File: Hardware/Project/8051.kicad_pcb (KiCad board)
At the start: 2 copper layers, 48 parts, among them J1 USB_B_Mini, J2 Conn_02x20_Odd_Even, Q1 9015, Q2 9013, SW1 reset, U1 8255, U10 74LS138, U11 74LS14, U12 74LS00, U13 STC89C52-Vintage, U14 74LS08, U18 74LS32, U19 74LS30, U2 74LS373_ARRANGED, U20 AT29C512, U21 74LS32, U22 74LS138, U5 74LS138, U6 28C256, U7 28C256, U9 ATA, Y2 Crystal

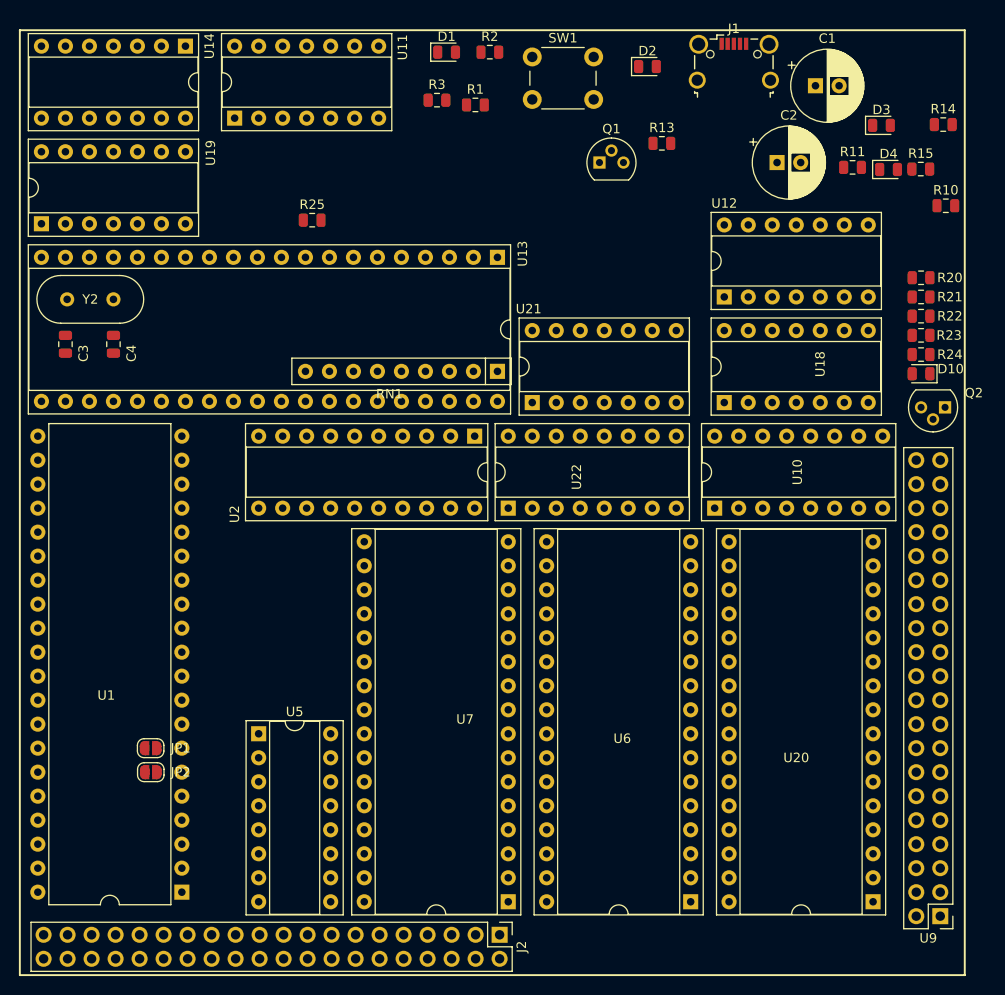
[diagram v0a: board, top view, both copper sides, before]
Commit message: 1
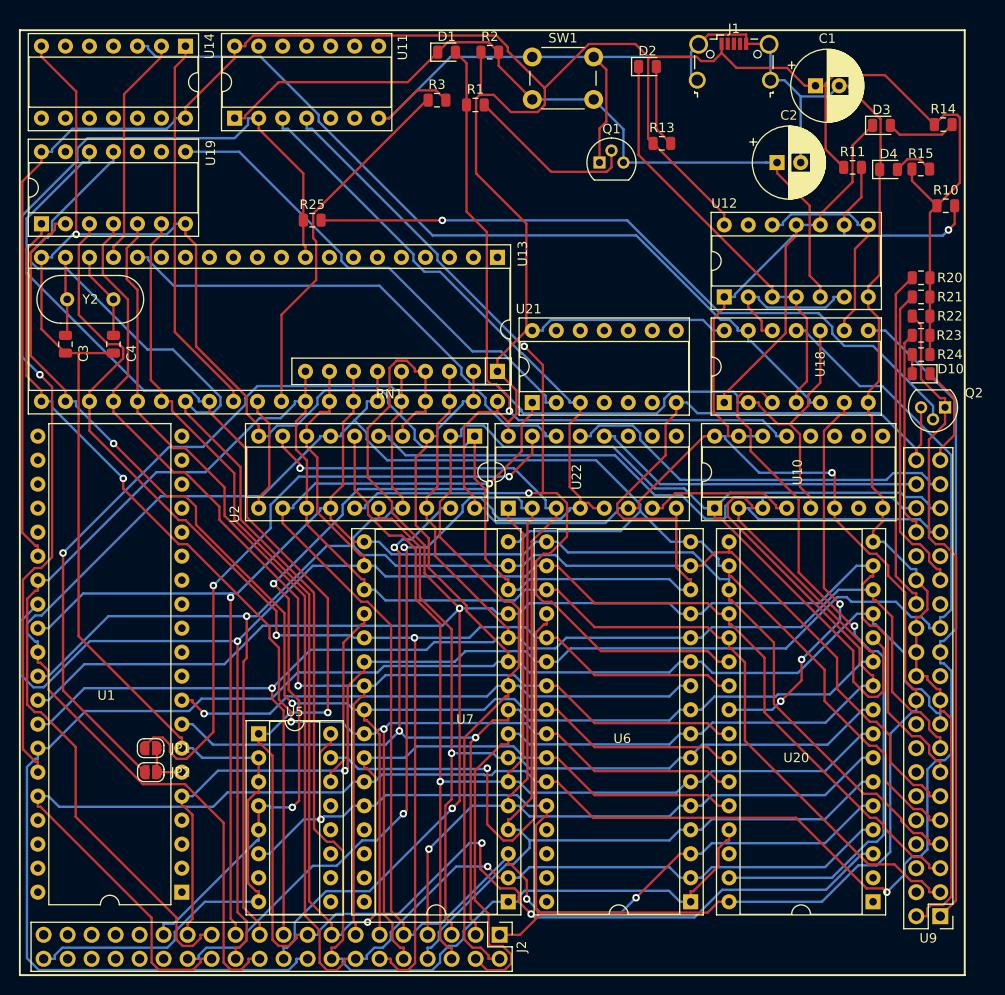
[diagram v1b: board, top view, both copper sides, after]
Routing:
- net /+5V: track 0.00 -> 506.3 mm, vias 0 -> 2
- net /GND: track 0.00 -> 502.7 mm, vias 0 -> 1
- net /~A0: track 0.00 -> 214.9 mm, vias 0 -> 1
- net /~D2: track 0.00 -> 214.0 mm, vias 0 -> 2
- net /~D0: track 0.00 -> 204.2 mm
- net /~D4: track 0.00 -> 203.5 mm
- net /~WR: track 0.00 -> 197.2 mm, vias 0 -> 1
- net /~D7: track 0.00 -> 194.2 mm
- net /~D6: track 0.00 -> 189.5 mm, vias 0 -> 1
- net /~A15: track 0.00 -> 187.3 mm, vias 0 -> 3
- net /~D3: track 0.00 -> 176.7 mm, vias 0 -> 1
- net /~D1: track 0.00 -> 175.3 mm, vias 0 -> 1
- net /~D5: track 0.00 -> 174.7 mm, vias 0 -> 1
- net /~A1: track 0.00 -> 173.7 mm, vias 0 -> 3
- net /~A2: track 0.00 -> 169.0 mm
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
